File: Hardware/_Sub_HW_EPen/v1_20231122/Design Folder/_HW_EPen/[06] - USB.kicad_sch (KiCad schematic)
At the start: 10 parts, among them J601 USB_microB_RA

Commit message: Hardware is almost done
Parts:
- J601: footprint Connector_USB:USB_Micro-B_Amphenol_10118194_Horizontal -> _PCBLIB_EPen:USB_Micro-B_Amphenol_10118194_Horizontal
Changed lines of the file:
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@@
       (effects (font (size 1.27 1.27)))
     )
-    (property "Footprint" "Connector_USB:USB_Micro-B_Amphenol_10118194_Horizontal" (at 128.27 106.68 0)
+    (property "Footprint" "_PCBLIB_EPen:USB_Micro-B_Amphenol_10118194_Horizontal" (at 128.27 106.68 0)
       (effects (font (size 1.27 1.27)) (justify left) hide)
     )

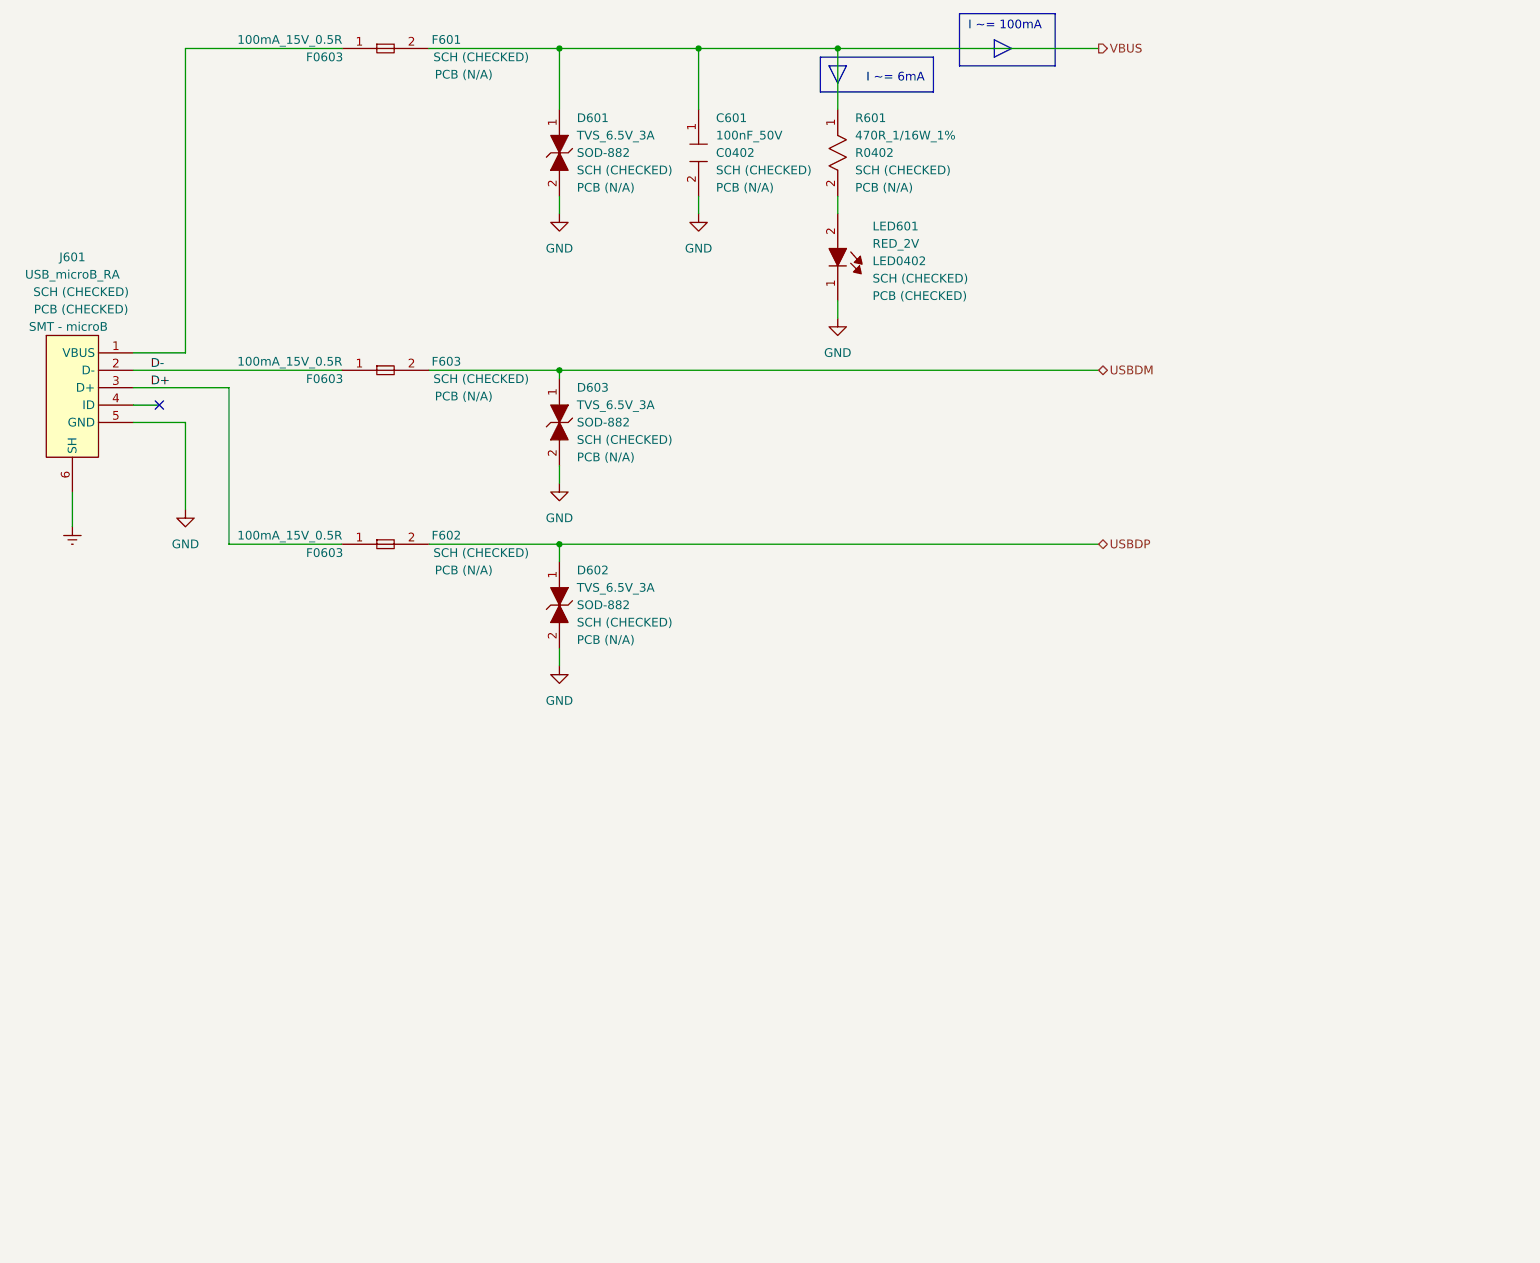
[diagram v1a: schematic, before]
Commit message: Updating file templates and structures...
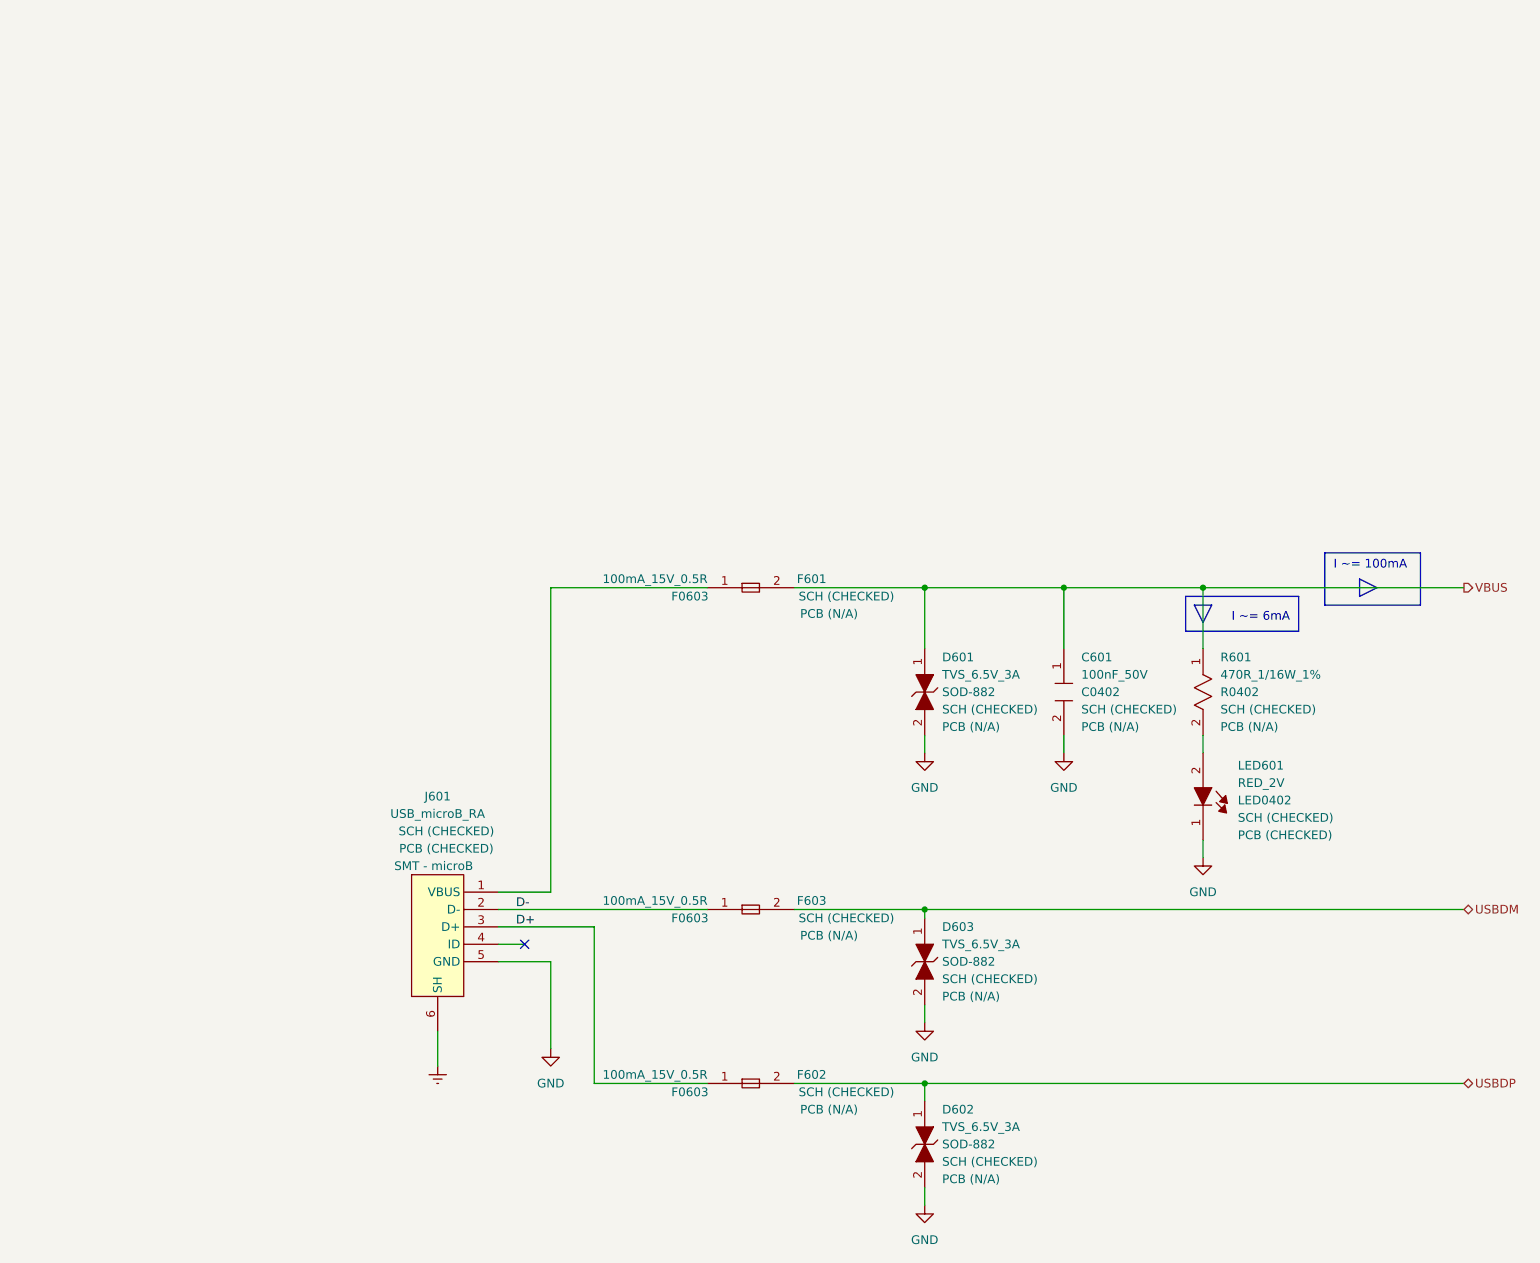
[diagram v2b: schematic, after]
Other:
- moved on the sheet: C601, D601, D602, D603, F601, F602, F603, J601, LED601, R601

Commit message: Updating Hardware File structures
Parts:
- C601: Manufacturer (none) -> Murata Electronics; Part Number GRM155R71H104KE14J -> (none); Part Number (Manufacturer) (none) -> GRM155R71H104KE14J; Part Number (Vendor) (none) -> 490-13342-2-ND; Vendor (none) -> Digikey
- D601, D602, D603: Manufacturer (none) -> Good-Ark Semiconductor; Part Number GSEWT5B003 -> (none); Part Number (Manufacturer) (none) -> GSEWT5B003; Part Number (Vendor) (none) -> 4786-GSEWT5B003TR-ND; Vendor (none) -> Digikey
- F601, F602, F603: Manufacturer (none) -> Eaton - Electronics Division; Part Number PTS060315V010 -> (none); Part Number (Manufacturer) (none) -> PTS060315V010; Part Number (Vendor) (none) -> 283-PTS060315V010TR-ND; Vendor (none) -> Digikey
- J601: Manufacturer (none) -> Amphenol ICC (FCI); Part Number 10118194-0001LF -> (none); Part Number (Manufacturer) (none) -> 10118194-0001LF; Part Number (Vendor) (none) -> 609-4618-2-ND; Vendor (none) -> Digikey
- LED601: Manufacturer (none) -> Harvatek Corporation; Part Number B2841USD-20D001014U1930 -> (none); Part Number (Manufacturer) (none) -> B2841USD-20D001014U1930; Part Number (Vendor) (none) -> 3147-B2841USD-20D001014U1930TR-ND; Vendor (none) -> Digikey
- R601: Manufacturer (none) -> Bourns Inc.; Part Number CR0402-FX-4700GLF -> (none); Part Number (Manufacturer) (none) -> CR0402-FX-4700GLF; Part Number (Vendor) (none) -> CR0402-FX-4700GLFTR-ND; Vendor (none) -> Digikey
